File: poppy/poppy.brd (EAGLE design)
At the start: 30 x 51 mm, 16 parts, among them Q1 10MHz, U1 ATUSB, U2 MBI5039

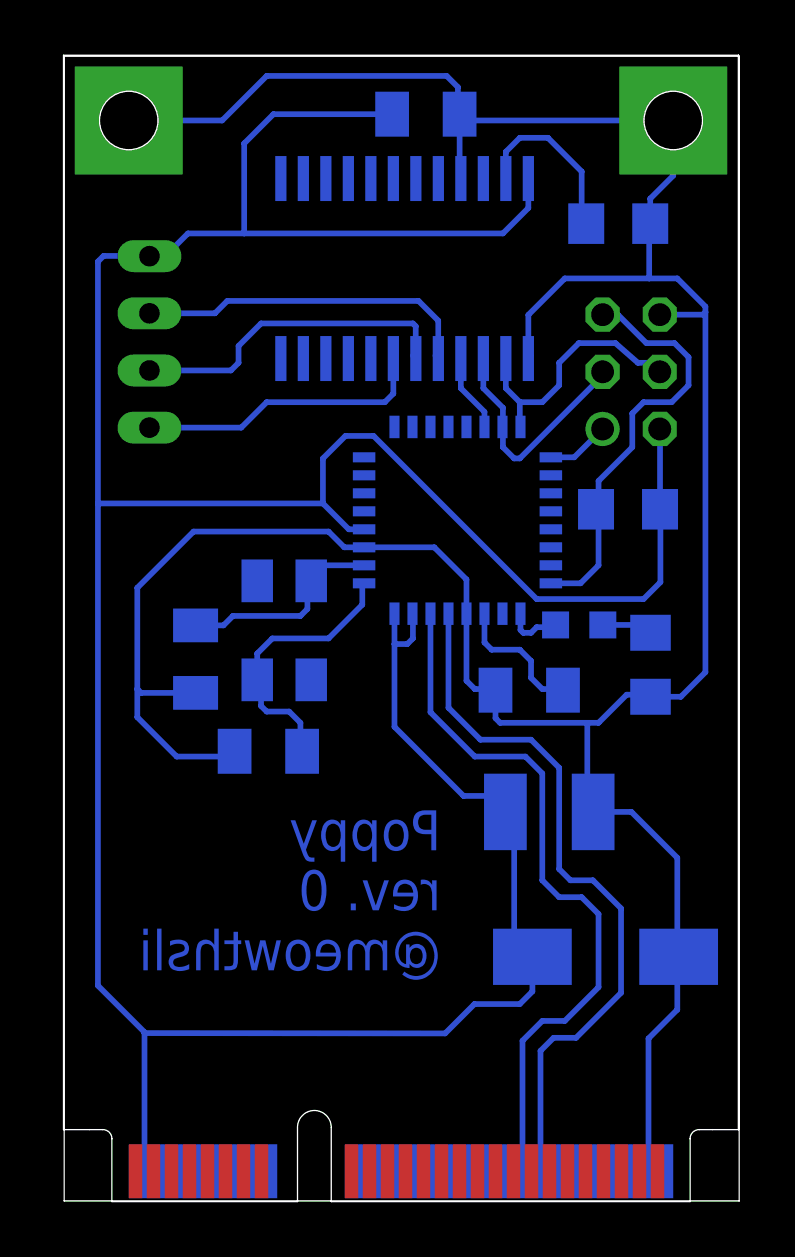
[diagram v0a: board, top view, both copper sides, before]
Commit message: Ready to solder
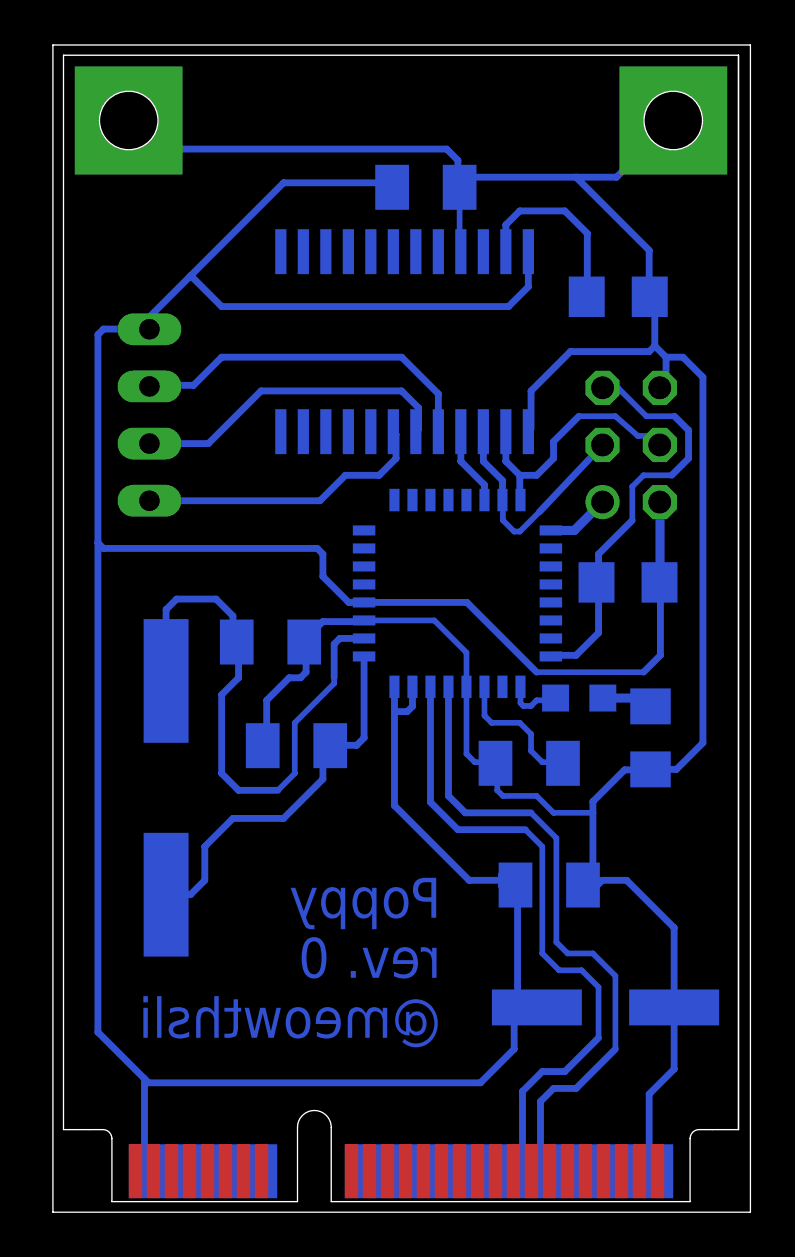
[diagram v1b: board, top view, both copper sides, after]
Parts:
- C1: device resistor:C4532 -> resistor:C1206K
- C2: value 47u -> 10u; device resistor:150CLZ-0810 -> resistor:153CLV-0807
- C5: value 4u7 -> 1u
- Q1: value 10MHz -> 8MHz; device crystal:CTS406 -> crystal:CSM-7X-DU
- R1, R2: device resistor:R1206 -> resistor:R3216
- R3: value 3k9 -> 1k; device resistor:R1206 -> resistor:R3216
- moved Q1 8.75 mm to (4.53, 18.4)
- moved C4 3.42 mm to (9.17, 24.8), turned to 180 degrees
- moved C1 3.25 mm to (21.6, 14.0)
- moved C5 3.25 mm to (20.7, 19.4)
- moved C6 3.25 mm to (16.1, 45.0)
- moved ISP 3.25 mm to (25.2, 33.6)
- moved LED1 3.25 mm to (22.9, 22.4)
- moved LED2 3.25 mm to (3.79, 34.9)
- moved R1 3.25 mm to (25.1, 27.5)
- moved R2 3.25 mm to (26.1, 20.6)
- moved R3 3.25 mm to (24.6, 40.2)
- moved U1 3.25 mm to (17.5, 27.0)
- moved U2 3.25 mm to (15.2, 38.3)
- moved C2 2.25 mm to (24.1, 8.60)
- moved C3 1.27 mm to (10.3, 20.2)
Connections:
- net XTAL2: now also Q1.2; no longer Q1.3
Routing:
- net GND: track 140.4 -> 124.3 mm
- net XTAL2: track 10.6 -> 25.9 mm
- net VCC: track 154.9 -> 148.4 mm
- net XTAL1: track 12.4 -> 16.9 mm
- net D+: track 31.9 -> 28.9 mm
- net D-: track 31.8 -> 29.0 mm
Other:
- board size 30 x 51 mm -> 31 x 51.9 mm
